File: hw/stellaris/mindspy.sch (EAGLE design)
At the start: 43 parts, among them IC1 ADS1298, IC3 MCP1703CB, X1 DF9-31S, X2 STELLARIS-LAUNCHPADSTELLARIS-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

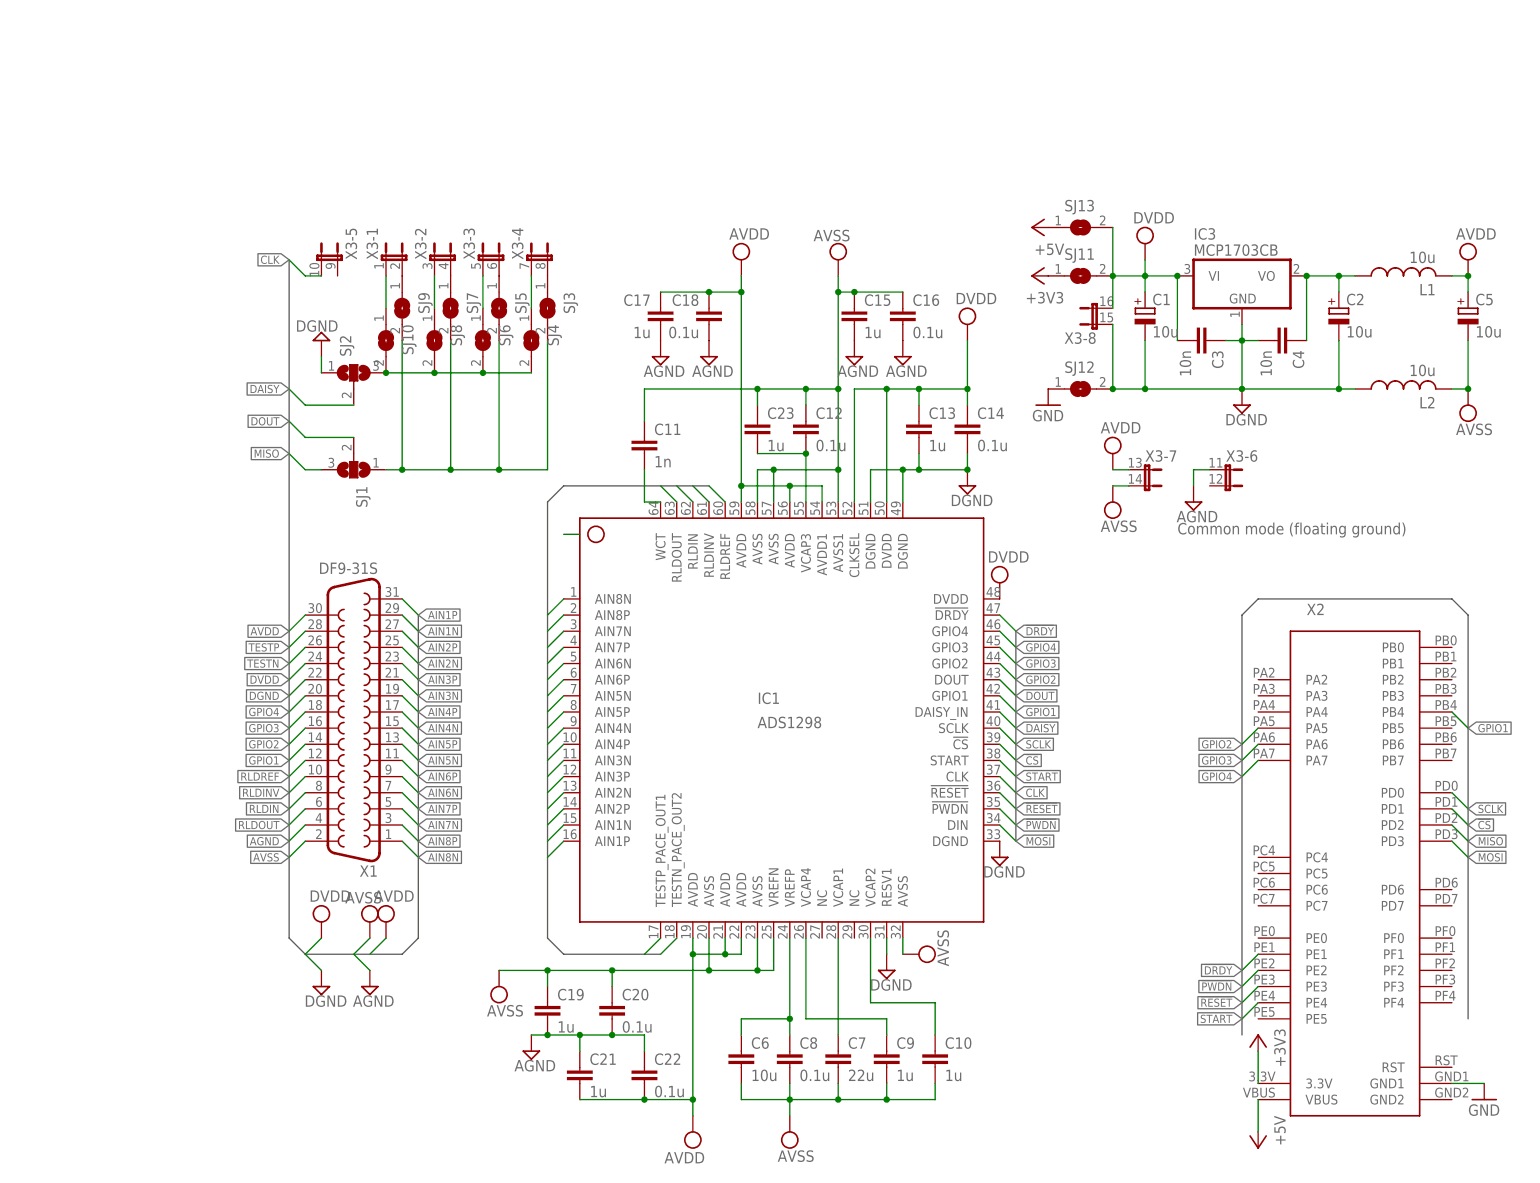
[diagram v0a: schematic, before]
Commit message: Major modifications.
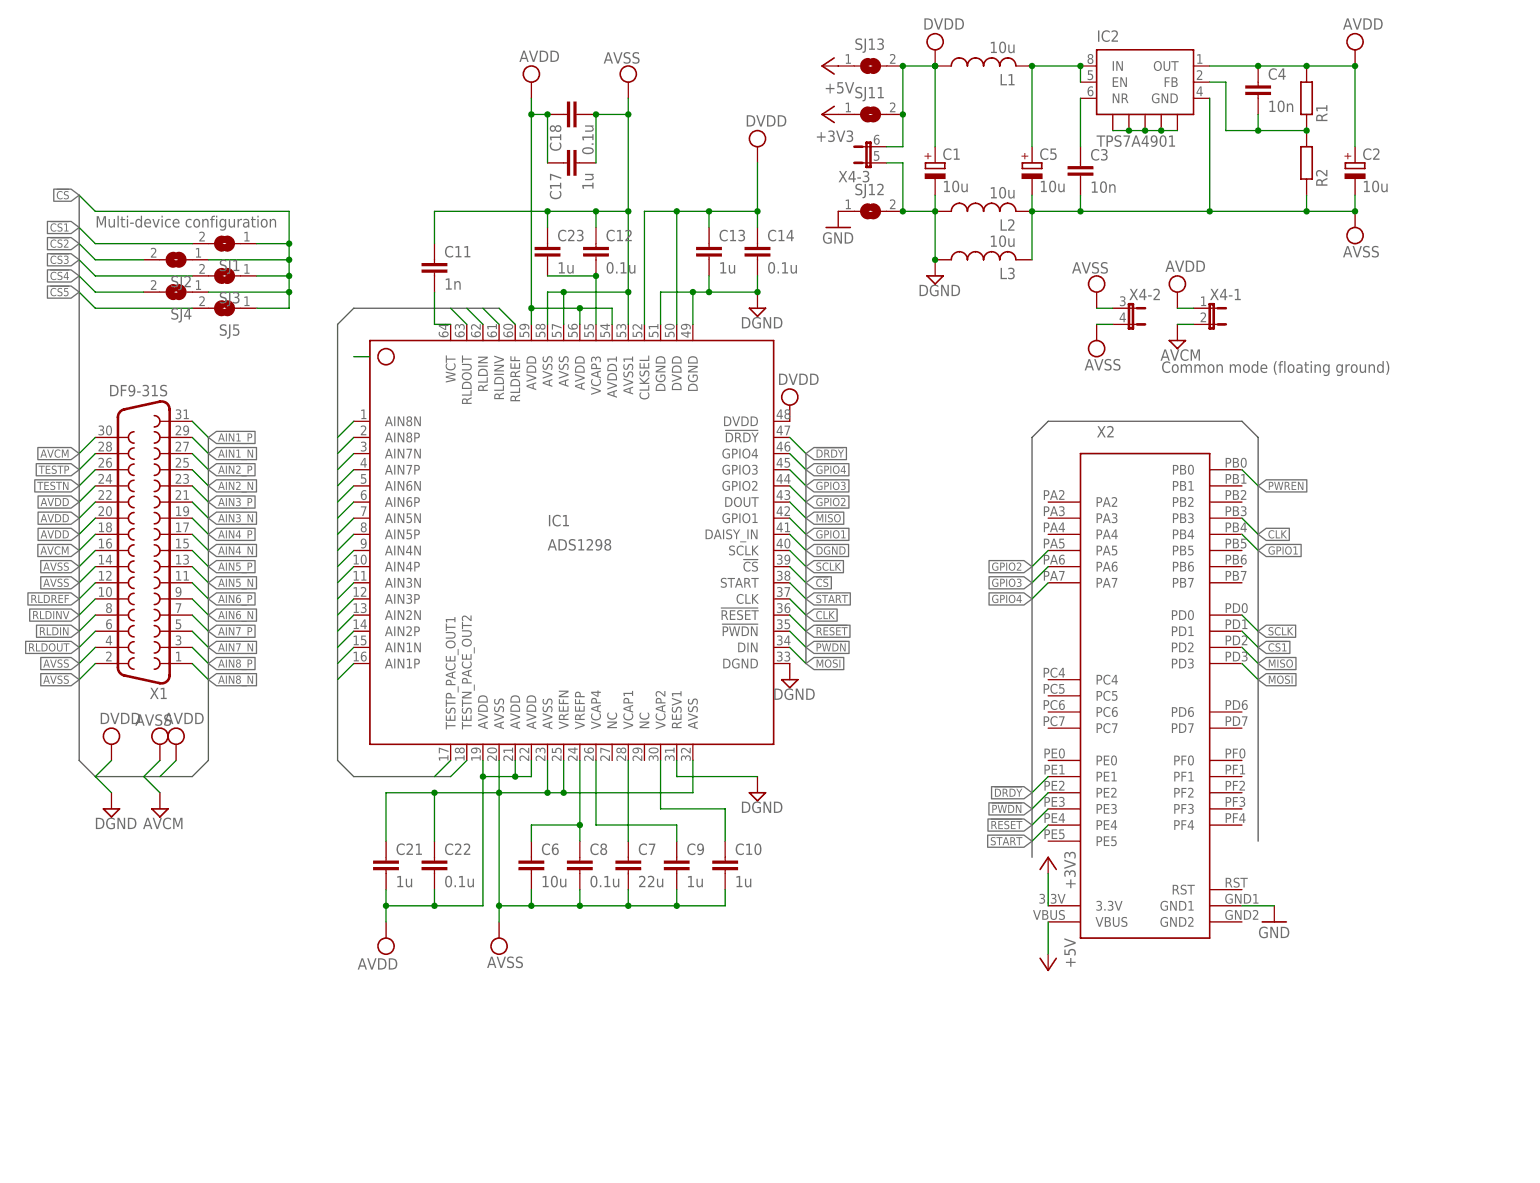
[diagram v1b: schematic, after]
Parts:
- removed C15, C19: 1u, rcl:C-EUC0805K
- removed C16, C20: 0.1u, rcl:C-EUC0603K
- removed IC3: MCP1703CB, linear:MCP1703CB
- removed SJ10, SJ6, SJ7, SJ8, SJ9: (no value), jumper:SJ
- removed X3: (no value), jumper:JP8QE
- added IC2: TPS7A4901, fabhack:TPS7A4901
- added L3: 10u, fabhack:L1210
- added R1, R2: (no value), rcl:R-EU_R0402
- added X4: (no value), jumper:JP3QE
- C1, C2, C5: device rcl:CPOL-EUSMCB -> rcl:CPOL-EUSMCA
- C10, C11, C12, C14, C18, C22, C8, C9: device rcl:C-EUC0603K -> rcl:C-EUC0402
- C13, C17, C21, C23: device rcl:C-EUC0805K -> rcl:C-EUC0402
- C3, C4: device rcl:C-EUC0603K -> rcl:C-EUC0603
- C6: device rcl:C-EUC0805K -> rcl:C-EUC0805
- C7: device rcl:C-EUC1206K -> rcl:C-EUC0805
- L1, L2: device rcl:L-USL1812 -> fabhack:L1210
- SJ1, SJ2: device jumper:SJ2W -> jumper:SJ
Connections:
- net AIN1N renamed AIN1_N
- net AIN1P renamed AIN1_P
- net AIN2N renamed AIN2_N
- net AIN2P renamed AIN2_P
- net AIN3N renamed AIN3_N
- net AIN3P renamed AIN3_P
- net AIN4N renamed AIN4_N
- net AIN4P renamed AIN4_P
- net AIN5N renamed AIN5_N
- net AIN5P renamed AIN5_P
- net AIN6N renamed AIN6_N
- net AIN6P renamed AIN6_P
- net AIN7N renamed AIN7_N
- net AIN7P renamed AIN7_P
- net AIN8N renamed AIN8_N
- net AIN8P renamed AIN8_P
- removed net AGND: C15.2, C16.2, C17.2, C18.2, C19.2, C20.2, C21.1, C22.1, X1.4, X3-6.1
- removed net DAISY: IC1.DAISY_IN, SJ2.2
- removed net DOUT: IC1.DOUT, SJ1.2
- removed net N$10: SJ7.1, X3-2.2
- removed net N$11: SJ6.1, X3-3.1
- removed net N$12: SJ5.1, X3-3.2
- removed net N$13: SJ8.1, X3-2.1
- removed net N$14: SJ3.1, X3-4.2
- removed net N$15: SJ10.1, X3-1.1
- removed net N$16: SJ10.2, SJ2.3, SJ4.2, SJ6.2, SJ8.2
- removed net N$18: SJ1.1, SJ3.2, SJ5.2, SJ7.2, SJ9.2
- removed net N$9: SJ4.1, X3-4.1
- new net !CS1: SJ1.2, X2.PD1
- new net !CS2: SJ2.2
- new net !CS3: SJ3.2
- new net !CS4: SJ4.2
- new net !CS5: SJ5.2
- new net AVCM: X1.18, X1.30, X4-1.2
- new net N$19: C4.2, IC2G$1.FB, R1.1, R2.2
- new net N$22: C5.+, IC2G$1.EN, IC2G$1.IN, L1.2
- new net PWREN: X2.PB0
- net !CS: now also SJ1.1, SJ2.1, SJ3.1, SJ4.1, SJ5.1; no longer X2.PD1
- net AVDD: now also C2.+, C4.1, IC2G$1.OUT, R1.2, X1.20, X1.22, X1.24, X4-1.1; no longer C5.+, L1.2, X1.30, X3-7.1
- net AVSS: now also C17.2, C18.2, C2.-, C21.1, C22.1, C3.2, IC2G$1.GND, L3.2, R2.1, X1.14, X1.16, X1.4, X4-2.1, X4-2.2; no longer C15.1, C16.1, C19.1, C20.1, X3-7.2
- net CLK: now also X2.PB3; no longer X3-5.2
- net DGND: now also IC1.DAISY_IN, L3.1, X4-3.1; no longer C2.-, C3.1, C4.2, IC3.GND, SJ2.1, X1.22, X3-8.1
- net DVDD: now also L1.1, X4-3.2; no longer C3.2, IC3.VI, X1.24, X3-8.2
- net GPIO1: no longer X1.14
- net GPIO2: no longer X1.16
- net GPIO3: no longer X1.18
- net GPIO4: no longer X1.20
- net MISO: now also IC1.DOUT; no longer SJ1.3
- net N$3: now also C3.1, IC2G$1.NR; no longer C2.+, C4.1, IC3.VO, L1.1
- net N$8: now also IC2G$2.GND, IC2G$2.GND@1, IC2G$2.GND@2, IC2G$2.GND@3, IC2G$2.GND@4; no longer SJ9.1, X3-1.2
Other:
- note added: "Multi-device configuration"
- moved on the sheet: C1, C10, C11, C12, C13, C14, C17, C18, C2, C21, C22, C23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
